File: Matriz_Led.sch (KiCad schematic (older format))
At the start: 18 parts, among them Q1 SMBT3904, Q2 SMBT3904, Q3 SMBT3904, Q4 SMBT3904, Q5 SMBT3904, U5 Matriz_5x7

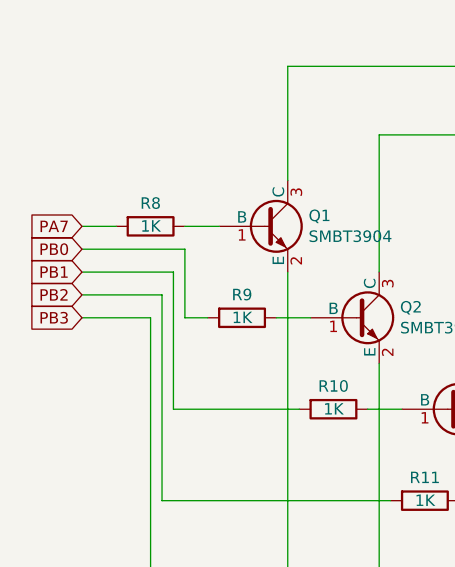
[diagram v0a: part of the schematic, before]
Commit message: finalizado enrutado provisional
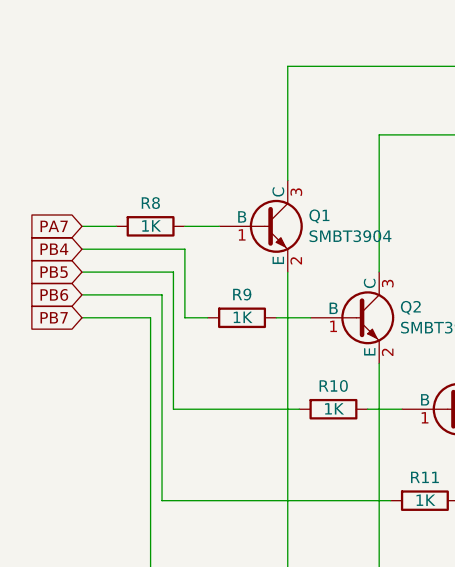
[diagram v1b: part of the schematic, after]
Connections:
- net PB0 renamed PB4
- net PB1 renamed PB5
- net PB2 renamed PB6
- net PB3 renamed PB7
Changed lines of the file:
@@
 PA7
 Text GLabel 2950 3850 0    50   Input ~ 0
-PB0
+PB4
 Text GLabel 2950 3950 0    50   Input ~ 0
-PB1
+PB5
 Text GLabel 2950 4050 0    50   Input ~ 0
-PB2
+PB6
 Text GLabel 2950 4150 0    50   Input ~ 0
-PB3
+PB7
 $EndSCHEMATC
